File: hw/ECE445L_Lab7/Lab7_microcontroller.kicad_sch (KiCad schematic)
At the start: 12 parts, among them J4 Debugger, SW6 RST, U4 M0G3507QDGS32RQ1, Y1 16MHz

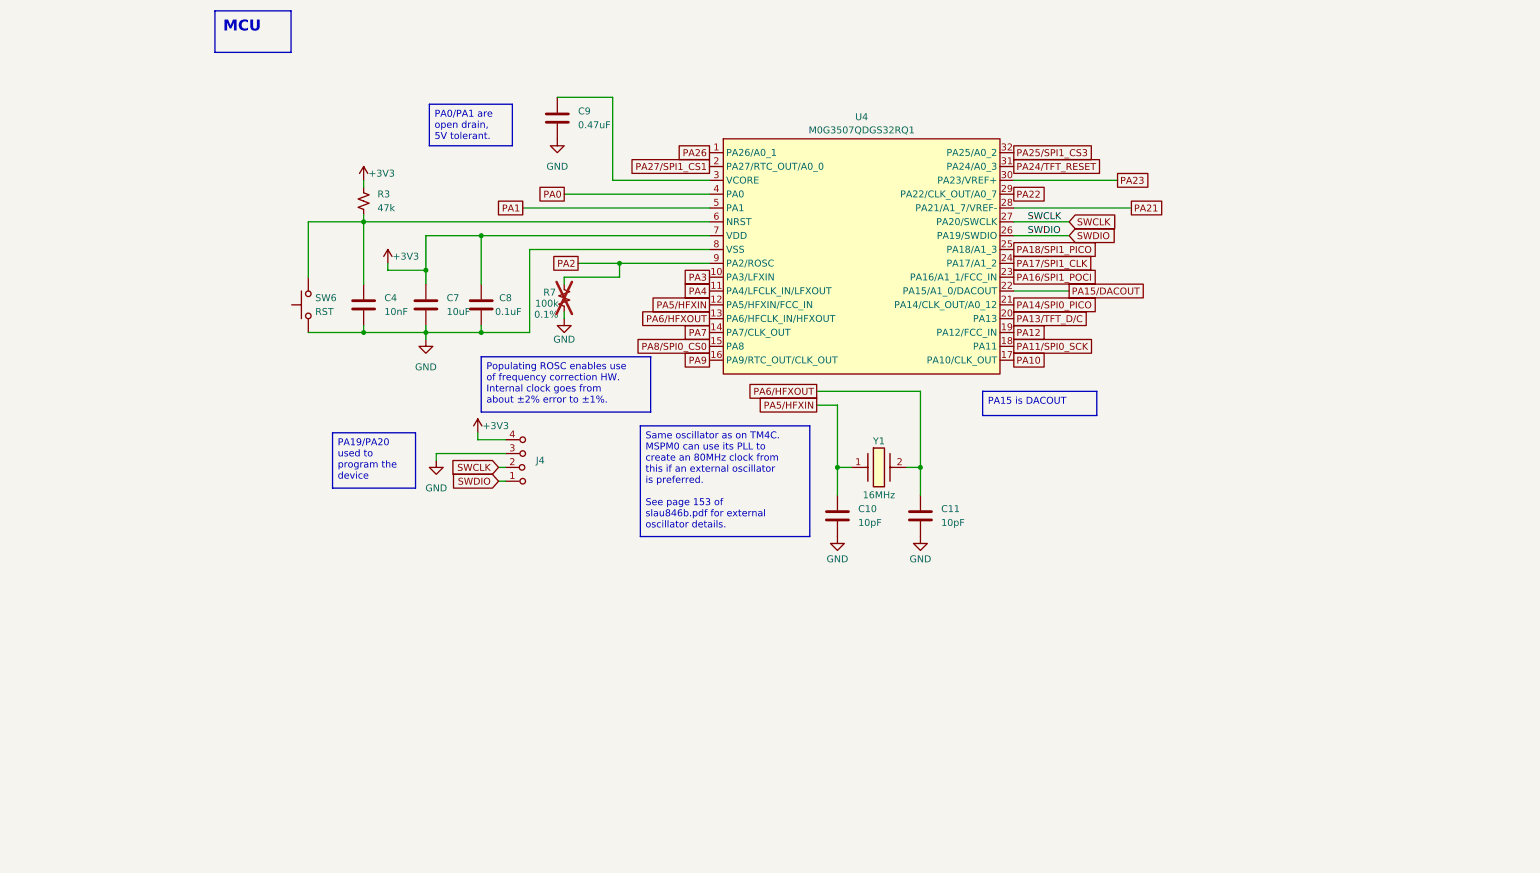
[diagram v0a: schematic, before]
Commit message: work on schem
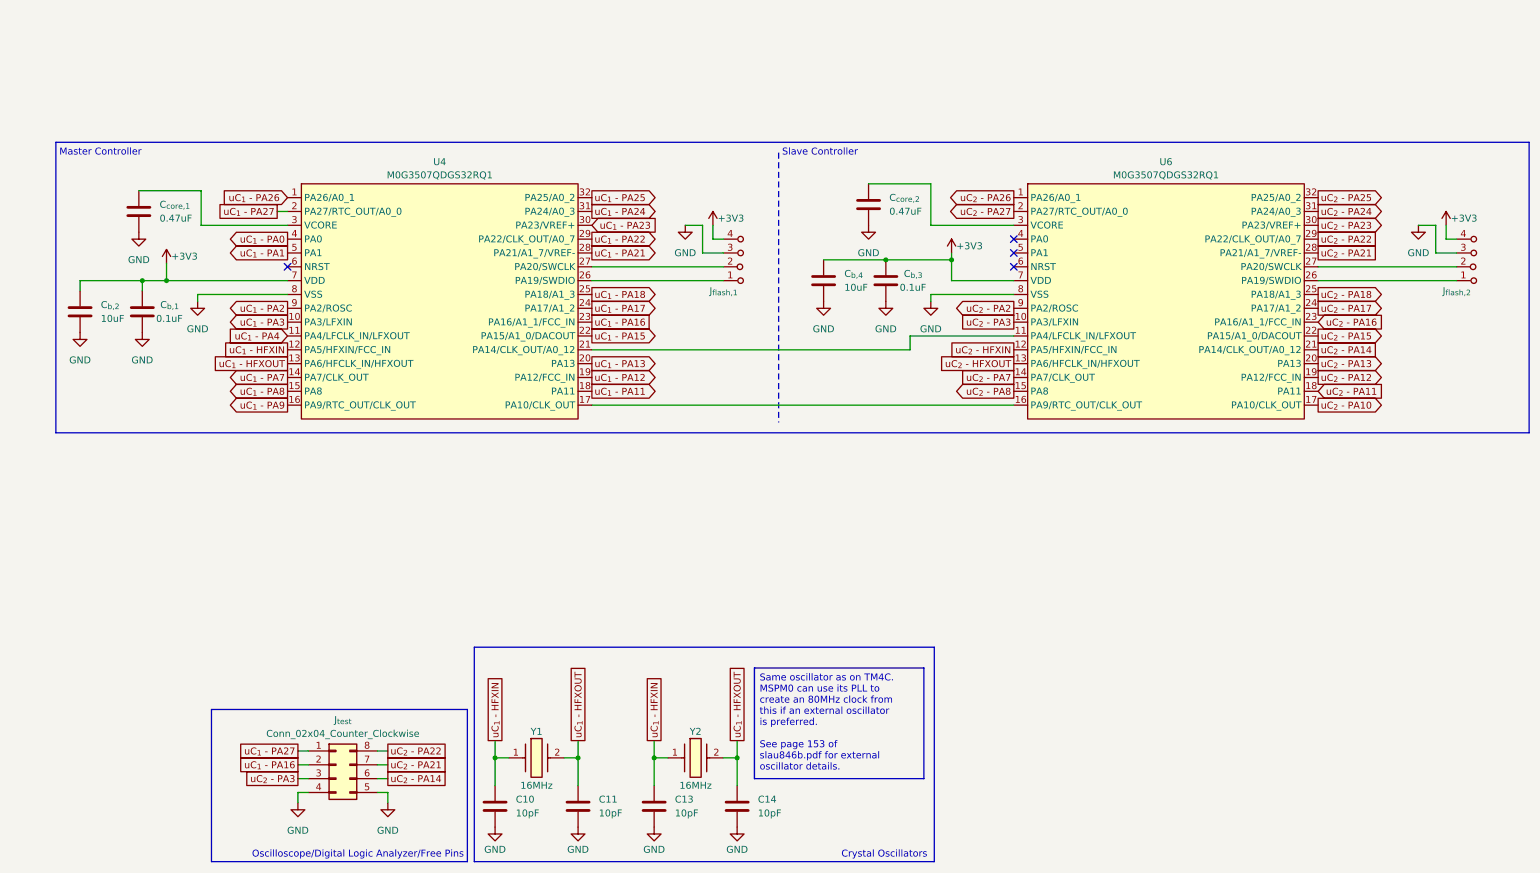
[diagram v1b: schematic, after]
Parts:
- removed C4: 10nF, ECE445L:C_Radial_100mil, symbol ECE445L:C
- removed R3: 47k, ECE445L:R_Axial_DIN0204_L3.6mm_D1.6mm_P7.62mm_Horizontal, symbol ECE445L:R_0.125W
- removed R7: 100k, ECE445L:R_Axial_DIN0204_L3.6mm_D1.6mm_P7.62mm_Horizontal, symbol ECE445L:R_0.125W
- removed SW6: RST, ECE445L:SW_PUSH_6mm, symbol ECE445L:SW_Push
- added C13, C14: 10pF, Capacitor_SMD:C_0201_0603Metric_Pad0.64x0.40mm_HandSolder, symbol ECE445L:C
- added C_{b,3}: 0.1uF, ECE445L:C_Radial_100mil, symbol ECE445L:C
- added C_{b,4}: 10uF, ECE445L:C_Radial_100mil, symbol ECE445L:C
- added C_{core,2}: 0.47uF, Capacitor_SMD:C_0201_0603Metric_Pad0.64x0.40mm_HandSolder, symbol ECE445L:C
- added J_{flash,2}: Debugger, ECE445L:PinHeader_1x04_P2.54mm_Vertical, symbol ECE445L:Header_4
- added J_{test}: Conn_02x04_Counter_Clockwise, Connector_PinSocket_2.54mm:PinSocket_2x04_P2.54mm_Vertical, symbol Connector_Generic:Conn_02x04_Counter_Clockwise
- added U6: M0G3507QDGS32RQ1, ECE445L:VSSOP_0.5mm_32pin_handsolder, symbol ECE445L:M0G3507QDGS32RQ1
- added Y2: 16MHz, ECE445L:ABM3, symbol ECE445L:ABM3-16.000MHZ-B2-T
- C10, C11: footprint ECE445L:C_Radial_100mil -> Capacitor_SMD:C_0201_0603Metric_Pad0.64x0.40mm_HandSolder
- C_{core,1}: renamed from C9; footprint ECE445L:C_Radial_100mil -> Capacitor_SMD:C_0201_0603Metric_Pad0.64x0.40mm_HandSolder
- renumbered C8 to C_{b,1}, C7 to C_{b,2}, J4 to J_{flash,1}
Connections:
- net +3V3: now also C_{b,3}.1, C_{b,4}.1, J_{flash,2}.4 (C), U6.7 (VDD)
- net GND: now also C13.2, C14.2, C_{b,3}.2, C_{b,4}.2, C_{core,2}.2, J_{flash,2}.3 (C), J_{test}.4 (Pin_4), J_{test}.5 (Pin_5), U6.8 (VSS)
- net PA0 renamed uC_{1} - PA0
- net PA1 renamed uC_{1} - PA1
- net PA10: no longer names the net of U4.17 (PA10/CLK_OUT)
- net PA10: now also U6.16 (PA9/RTC_OUT/CLK_OUT)
- net PA11/SPI0_SCK renamed uC_{1} - PA11
- net PA12 renamed uC_{1} - PA12
- net PA13/TFT_D/C renamed uC_{1} - PA13
- net PA14/SPI0_PICO: no longer names the net of U4.21 (PA14/CLK_OUT/A0_12)
- net PA14/SPI0_PICO: now also U6.11 (PA4/LFCLK_IN/LFXOUT)
- net PA15/DACOUT renamed uC_{1} - PA15
- net PA16/SPI1_POCI renamed uC_{1} - PA16
- net uC_{1} - PA16: now also J_{test}.2 (Pin_2)
- net PA17/SPI1_CLK renamed uC_{1} - PA17
- net PA18/SPI1_PICO renamed uC_{1} - PA18
- net PA2 renamed uC_{1} - PA2
- net PA21 renamed uC_{1} - PA21
- net PA22 renamed uC_{1} - PA22
- net PA23 renamed uC_{1} - PA23
- net PA24/TFT_RESET renamed uC_{1} - PA24
- net PA25/SPI1_CS3 renamed uC_{1} - PA25
- net PA26 renamed uC_{1} - PA26
- net PA27/SPI1_CS1 renamed uC_{1} - PA27
- net uC_{1} - PA27: now also J_{test}.1 (Pin_1)
- net PA3 renamed uC_{1} - PA3
- net PA4 renamed uC_{1} - PA4
- net PA5/HFXIN renamed uC_{1} - HFXIN
- net uC_{1} - HFXIN: now also C13.1, Y2.1
- net PA6/HFXOUT renamed uC_{1} - HFXOUT
- net uC_{1} - HFXOUT: now also C14.1, Y2.2
- net PA7 renamed uC_{1} - PA7
- net PA8/SPI0_CS0 renamed uC_{1} - PA8
- net PA9 renamed uC_{1} - PA9
- net SWCLK: no longer names the net of J_{flash,1}.2 (B), U4.27 (PA20/SWCLK)
- net SWDIO: no longer names the net of J_{flash,1}.1 (A), U4.26 (PA19/SWDIO)
- new net: J_{flash,2}.1 (A), U6.26 (PA19/SWDIO)
- new net: J_{flash,2}.2 (B), U6.27 (PA20/SWCLK)
- new net: C_{core,2}.1, U6.3 (VCORE)
- new net uC_{2} - HFXIN: U6.12 (PA5/HFXIN/FCC_IN)
- new net uC_{2} - HFXOUT: U6.13 (PA6/HFCLK_IN/HFXOUT)
- new net uC_{2} - PA10: U6.17 (PA10/CLK_OUT)
- new net uC_{2} - PA11: U6.18 (PA11)
- new net uC_{2} - PA12: U6.19 (PA12/FCC_IN)
- new net uC_{2} - PA13: U6.20 (PA13)
- new net uC_{2} - PA14: J_{test}.6 (Pin_6), U6.21 (PA14/CLK_OUT/A0_12)
- new net uC_{2} - PA15: U6.22 (PA15/A1_0/DACOUT)
- new net uC_{2} - PA16: U6.23 (PA16/A1_1/FCC_IN)
- new net uC_{2} - PA17: U6.24 (PA17/A1_2)
- new net uC_{2} - PA18: U6.25 (PA18/A1_3)
- new net uC_{2} - PA2: U6.9 (PA2/ROSC)
- new net uC_{2} - PA21: J_{test}.7 (Pin_7), U6.28 (PA21/A1_7/VREF-)
- new net uC_{2} - PA22: J_{test}.8 (Pin_8), U6.29 (PA22/CLK_OUT/A0_7)
- new net uC_{2} - PA23: U6.30 (PA23/VREF+)
- new net uC_{2} - PA24: U6.31 (PA24/A0_3)
- new net uC_{2} - PA25: U6.32 (PA25/A0_2)
- new net uC_{2} - PA26: U6.1 (PA26/A0_1)
- new net uC_{2} - PA27: U6.2 (PA27/RTC_OUT/A0_0)
- new net uC_{2} - PA3: J_{test}.3 (Pin_3), U6.10 (PA3/LFXIN)
- new net uC_{2} - PA7: U6.14 (PA7/CLK_OUT)
- new net uC_{2} - PA8: U6.15 (PA8)
- no-connect marks 0 -> 4
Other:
- note added: "Crystal Oscillators"
- note added: "Master Controller"
- note added: "Oscilloscope/Digital Logic Analyzer/Free Pins"
- note added: "Slave Controller"
- company: (none) -> ECE445L Lab 7
- title: (none) -> MCU
- moved on the sheet: C10, C11, C_{b,1}, C_{b,2}, C_{core,1}, J_{flash,1}, U4, Y1

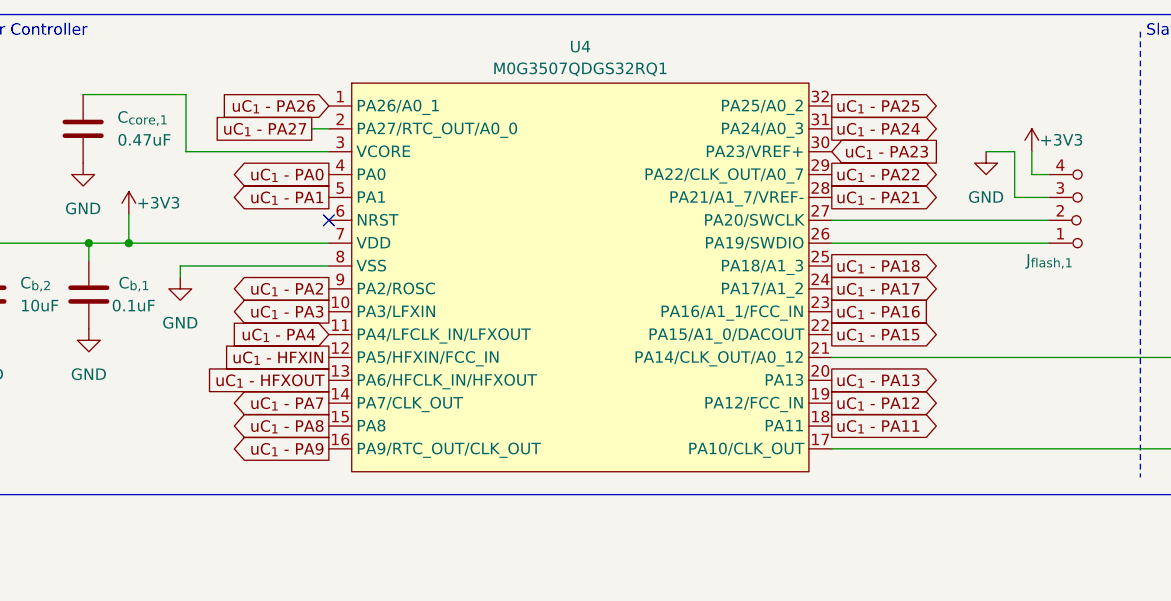
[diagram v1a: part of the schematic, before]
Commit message: more updates
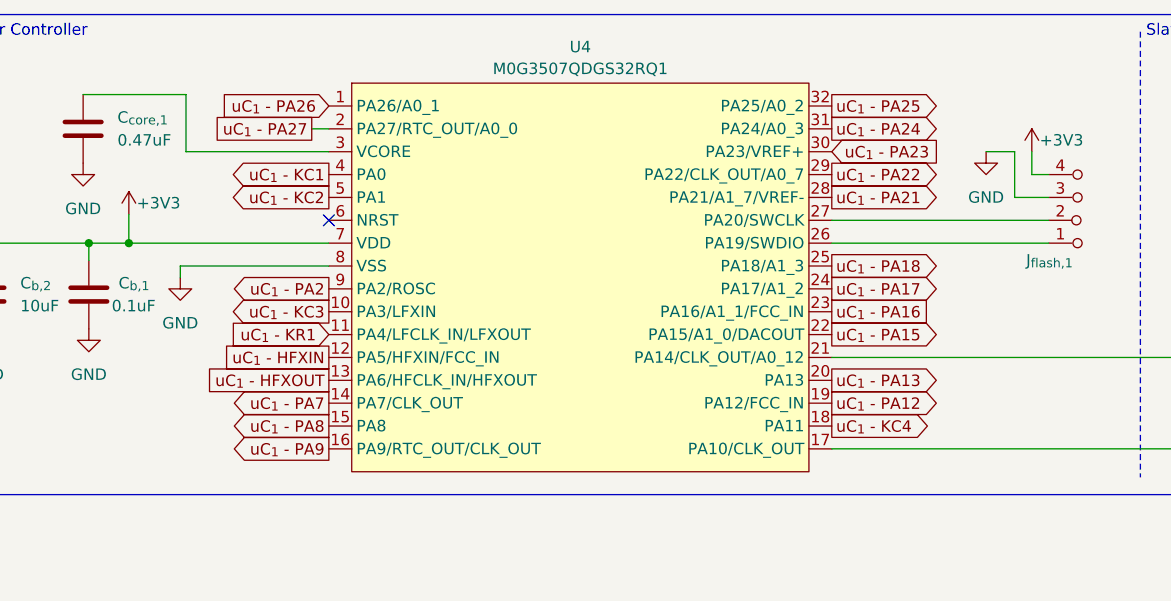
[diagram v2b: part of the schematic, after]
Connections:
- net uC_{1} - PA0 renamed uC_{1} - KC1
- net uC_{1} - PA1 renamed uC_{1} - KC2
- net uC_{1} - PA11 renamed uC_{1} - KC4
- net uC_{1} - PA3 renamed uC_{1} - KC3
- net uC_{1} - PA4 renamed uC_{1} - KR1
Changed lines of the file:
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@@
 		)
 	)
-	(global_label "uC_{1} - PA1"
+	(global_label "uC_{1} - KC2"
 		(shape output)
 		(at 56.515 84.455 180)
@@
 		)
 		(property "Intersheetrefs" "${INTERSHEET_REFS}"
-			(at 43.0675 84.455 0)
+			(at 42.8861 84.455 0)
 			(hide yes)
 			(show_name no)
@@
 		)
 	)
-	(global_label "uC_{1} - PA3"
+	(global_label "uC_{1} - KC3"
 		(shape output)
 		(at 56.515 97.155 180)
@@
 		)
 		(property "Intersheetrefs" "${INTERSHEET_REFS}"
-			(at 43.0675 97.155 0)
-			(hide yes)
-			(show_name no)
-			(do_not_autoplace no)
-			(effects
-				(font
-					(size 1.27 1.27)
-				)
-				(justify right)
-			)
-		)
-	)
-	(global_label "uC_{1} - PA4"
+			(at 42.8861 97.155 0)
+			(hide yes)
+			(show_name no)
+			(do_not_autoplace no)
+			(effects
+				(font
+					(size 1.27 1.27)
+				)
+				(justify right)
+			)
+		)
+	)
+	(global_label "uC_{1} - KR1"
 		(shape input)
 		(at 56.515 99.695 180)
@@
 		)
 		(property "Intersheetrefs" "${INTERSHEET_REFS}"
-			(at 43.0675 99.695 0)
-			(hide yes)
-			(show_name no)
-			(do_not_autoplace no)
-			(effects
-				(font
-					(size 1.27 1.27)
-				)
-				(justify right)
-			)
-		)
-	)
-	(global_label "uC_{1} - PA11"
+			(at 42.8861 99.695 0)
+			(hide yes)
+			(show_name no)
+			(do_not_autoplace no)
+			(effects
+				(font
+					(size 1.27 1.27)
+				)
+				(justify right)
+			)
+		)
+	)
+	(global_label "uC_{1} - KC4"
 		(shape output)
 		(at 112.395 109.855 0)
@@
 		)
 		(property "Intersheetrefs" "${INTERSHEET_REFS}"
-			(at 127.052 109.855 0)
+			(at 126.0239 109.855 0)
 			(hide yes)
 			(show_name no)
@@
 		)
 	)
-	(global_label "uC_{1} - PA0"
+	(global_label "uC_{1} - KC1"
 		(shape output)
 		(at 56.515 81.915 180)
@@
 		)
 		(property "Intersheetrefs" "${INTERSHEET_REFS}"
-			(at 43.0675 81.915 0)
-			(hide yes)
-			(show_name no)
+			(at 42.8861 81.915 0)
+			(hide yes)
+			(show_name no)

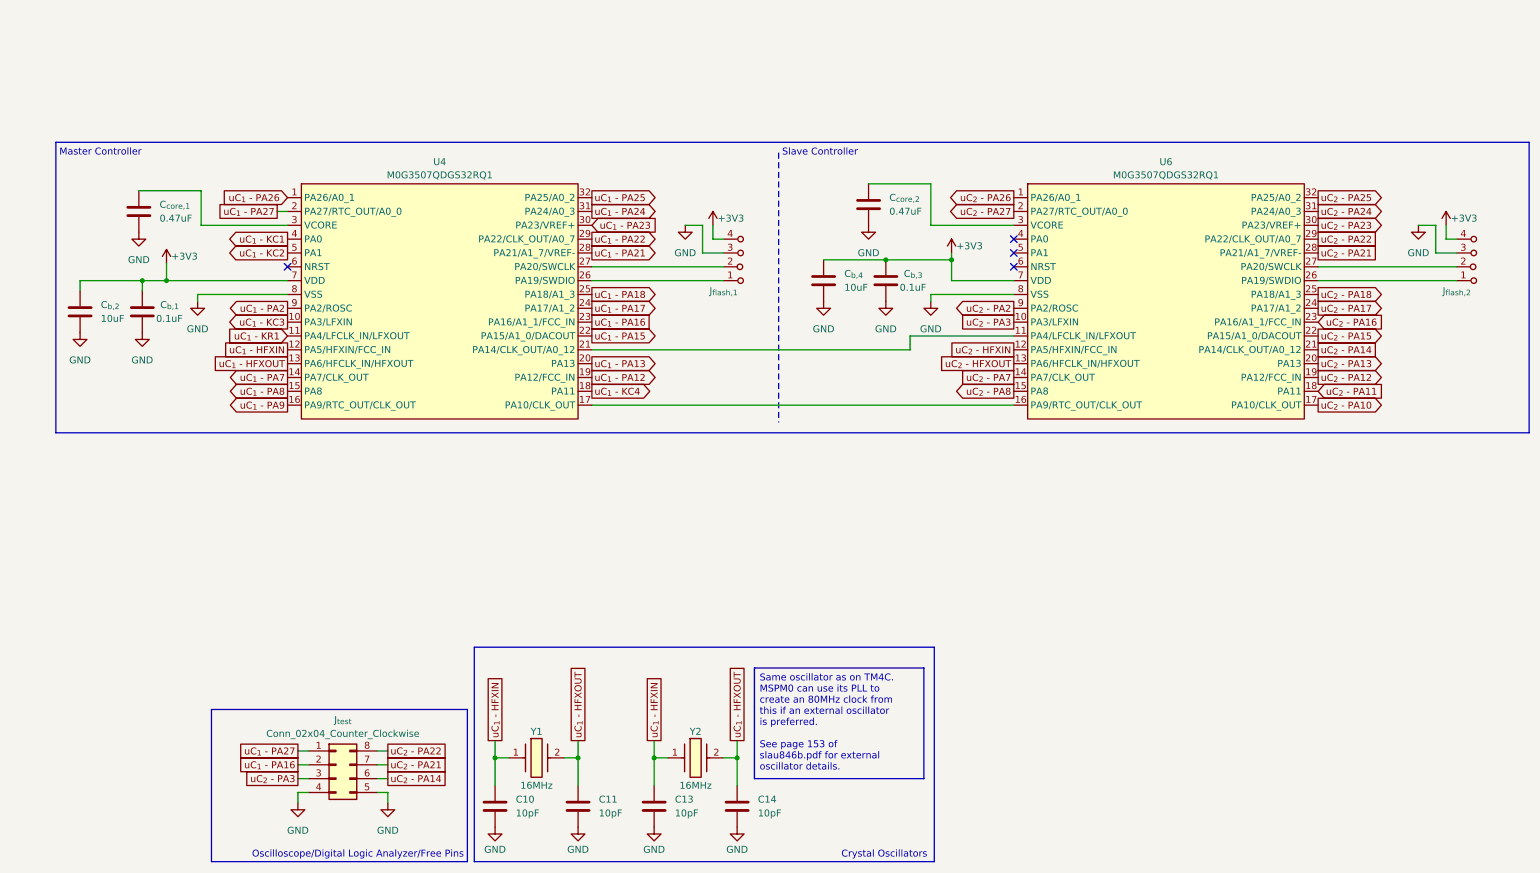
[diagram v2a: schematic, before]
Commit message: mostly finished schem
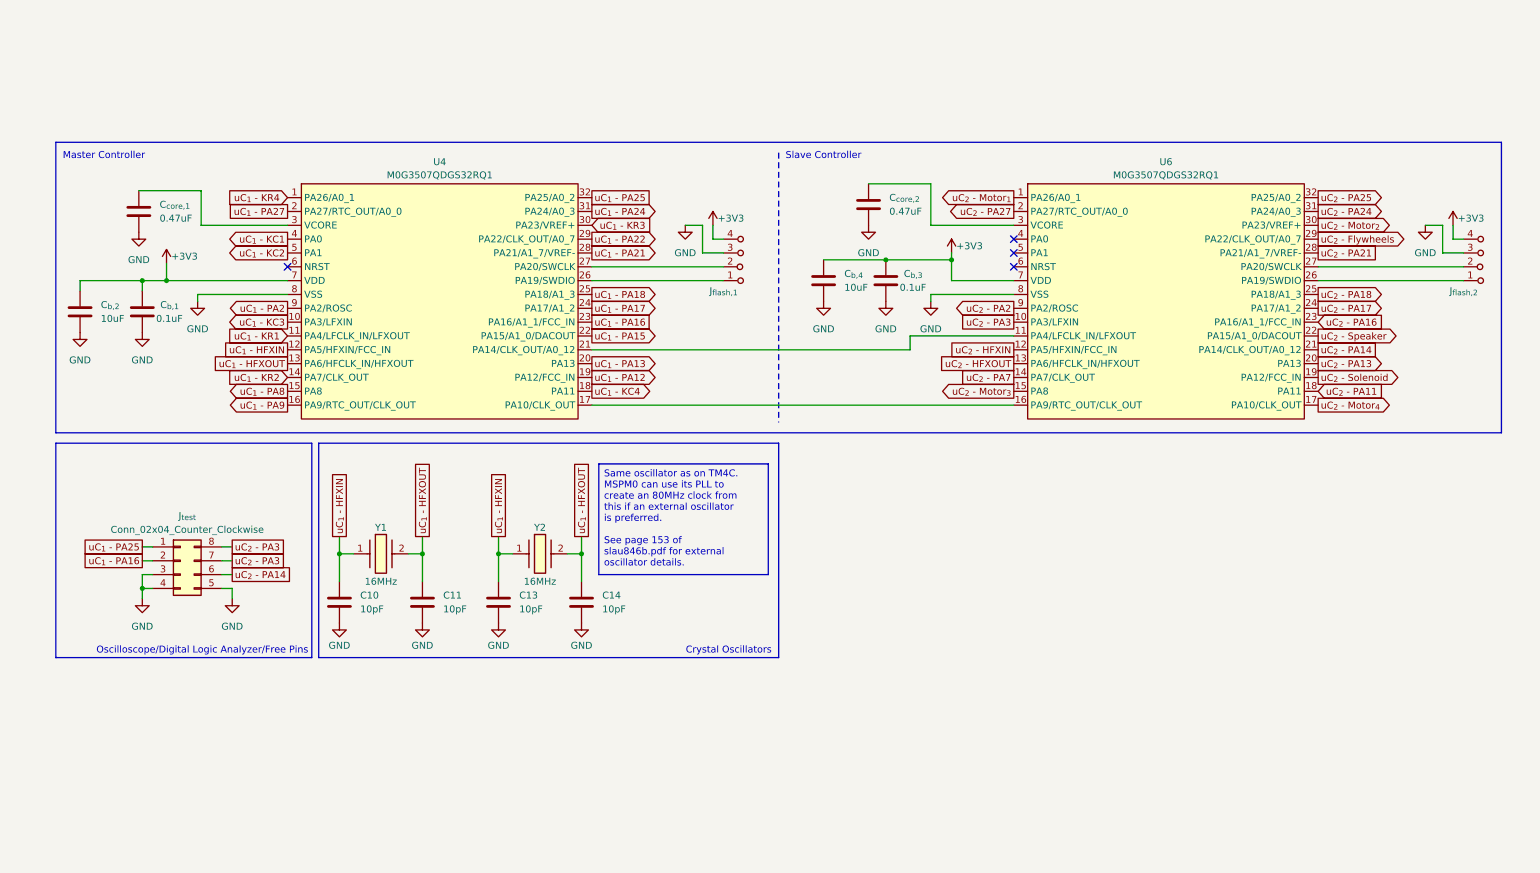
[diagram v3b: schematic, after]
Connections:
- net GND: now also J_{test}.3 (Pin_3)
- net uC_{1} - PA25: now also J_{test}.1 (Pin_1)
- net uC_{1} - PA27: no longer J_{test}.1 (Pin_1)
- net uC_{2} - PA21: no longer J_{test}.7 (Pin_7)
- net uC_{2} - PA3: now also J_{test}.7 (Pin_7), J_{test}.8 (Pin_8); no longer J_{test}.3 (Pin_3)
- net uC_{1} - PA23 renamed uC_{1} - KR3
- net uC_{1} - PA26 renamed uC_{1} - KR4
- net uC_{1} - PA7 renamed uC_{1} - KR2
- net uC_{2} - PA10 renamed uC_{2} - Motor_{4}
- net uC_{2} - PA12 renamed uC_{2} - Solenoid
- net uC_{2} - PA15 renamed uC_{2} - Speaker
- net uC_{2} - PA22 renamed uC_{2} - Flywheels
- net uC_{2} - Flywheels: no longer J_{test}.8 (Pin_8)
- net uC_{2} - PA23 renamed uC_{2} - Motor_{2}
- net uC_{2} - PA26 renamed uC_{2} - Motor_{1}
- net uC_{2} - PA8 renamed uC_{2} - Motor_{3}
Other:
- moved on the sheet: C10, C11, C13, C14, J_{flash,2}, J_{test}, Y1, Y2
